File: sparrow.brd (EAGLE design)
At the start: 80 x 80 mm, 201 parts, among them IC1 LAN8720AVIAS, IC2 TLV320AIC3100VIAS, IC3 TPS2500, IC4 SKYWORKS_AAT4280ASC70JW-8-NOT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, IC5 SKYWORKS_AAT4280ASC70JW-8-NOT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, IC6 SKYWORKS_AAT4280ASC70JW-8-NOT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, IC7 SKYWORKS_AAT4280ASC70JW-8-NOT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, IC8 SKYWORKS_AAT4280ASC70JW-8-NOT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, IC9 FXMA10820-DFN, X1 ABS07-32768, X2 12MHz, X3 32768, X4 50MHZ, X5 16MHz

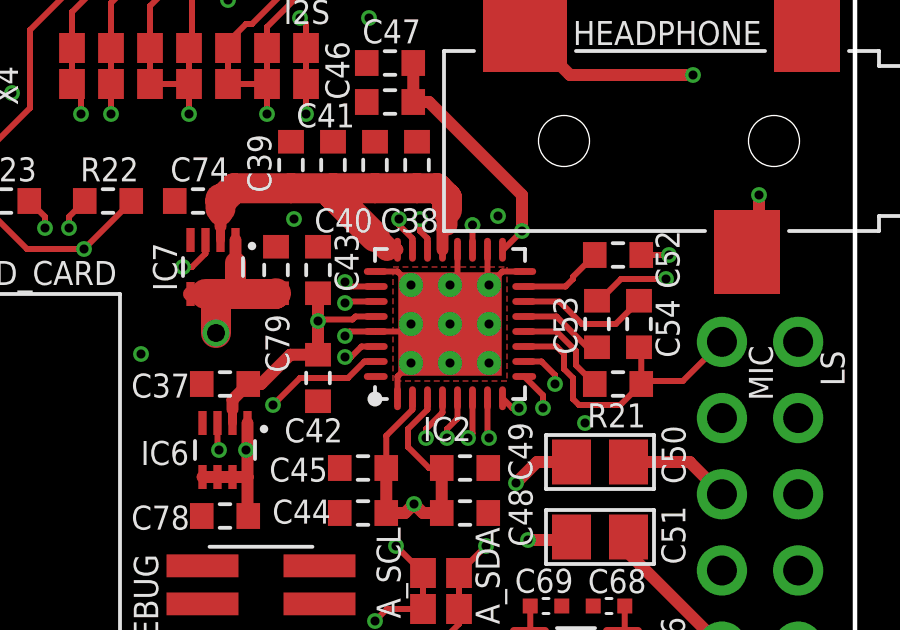
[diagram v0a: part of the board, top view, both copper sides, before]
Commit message: Last library update, DRC fixes
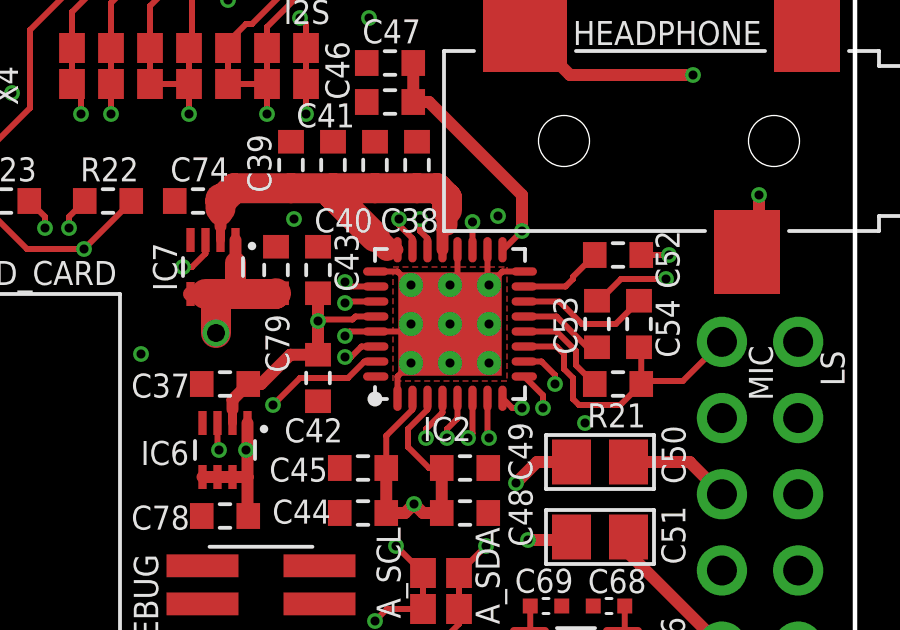
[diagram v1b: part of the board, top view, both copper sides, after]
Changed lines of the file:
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@@
 <contactref element="IC2" pad="19"/>
 <contactref element="LS" pad="2"/>
-<wire x1="67.25" y1="30.375" x2="67.25" y2="31.2" width="0.2" layer="1"/>
-<via x="67.25" y="31.2" extent="1-16" drill="0.3"/>
+<wire x1="67.25" y1="30.375" x2="67.25" y2="31.3" width="0.2" layer="1"/>
+<via x="67.25" y="31.3" extent="1-16" drill="0.3"/>
 <via x="64.8" y="31.4" extent="1-16" drill="0.3"/>
 <wire x1="65.25" y1="30.375" x2="65.25" y2="30.75" width="0.2" layer="1"/>
@@
 <wire x1="64.8" y1="31" x2="65.4" y2="30.4" width="0.4" layer="2"/>
 <wire x1="65.4" y1="30.4" x2="66.45" y2="30.4" width="0.4" layer="2"/>
-<wire x1="66.45" y1="30.4" x2="67.25" y2="31.2" width="0.4" layer="2"/>
 <wire x1="67.8" y1="32.2" x2="67.25" y2="31.65" width="0.4" layer="15"/>
-<wire x1="67.25" y1="31.65" x2="67.25" y2="31.2" width="0.4" layer="15"/>
+<wire x1="67.25" y1="31.65" x2="67.25" y2="31.3" width="0.4" layer="15"/>
 <wire x1="73.6" y1="31.8" x2="68.9" y2="31.8" width="0.4" layer="15"/>
 <wire x1="68.9" y1="31.8" x2="68.5" y2="32.2" width="0.4" layer="15"/>
@@
 <wire x1="76.8" y1="28.6" x2="76.8" y2="26.07" width="0.4" layer="15"/>
 <wire x1="76.8" y1="26.07" x2="78.105" y2="24.765" width="0.4" layer="15"/>
+<wire x1="66.45" y1="30.4" x2="67.25" y2="31.2" width="0.4" layer="2"/>
+<wire x1="67.25" y1="31.2" x2="67.25" y2="31.3" width="0.4" layer="2"/>
 </signal>
 <signal name="HPR">
@@
 <contactref element="MCLK" pad="2"/>
 <wire x1="68.25" y1="25.425" x2="68.575" y2="25.1" width="0.2" layer="1"/>
-<wire x1="68.575" y1="25.1" x2="68.8" y2="25.1" width="0.2" layer="1"/>
-<via x="68.8" y="25.1" extent="1-16" drill="0.3"/>
-<wire x1="68.8" y1="25.1" x2="67.7" y2="25.1" width="0.2" layer="15"/>
+<wire x1="68.575" y1="25.1" x2="68.9" y2="25.1" width="0.2" layer="1"/>
+<via x="68.9" y="25.1" extent="1-16" drill="0.3"/>
+<wire x1="68.9" y1="25.1" x2="67.7" y2="25.1" width="0.2" layer="15"/>
 <wire x1="67.7" y1="25.1" x2="67" y2="25.8" width="0.2" layer="15"/>
 <wire x1="67" y1="25.8" x2="63.2" y2="25.8" width="0.2" layer="15"/>

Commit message: Updated values
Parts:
- C10, C8, C9: value 4µ7 -> 4.7u
- C27, C52, C53, C56, C76, C77, C78, C79, C80: value 1µ -> 1u
- C29, C42, C44, C46, C48, L1: value 10µ -> 10u
- C40, C41: value 22µ -> 22u
- C50, C51: value 47µ -> 47u
- C55: value 2p2 -> 2.2p
- C57, C59: value 22µ 10V -> 22u 10V
- C60: value 150µ 10V -> 150u 10V
- C72, L5: value 2n2 -> 2.2n
- L7: value 2µ2 -> 2.2u
- R1: value 768k -> 768K
- R10, R11, R12, R13, R8, R9: value 12K -> 10K
- R16: value 12K1 -> 12.1K
- R17, R18, R19, R20: value 49R9 -> 49.9 1%
- R2: value 2M4 -> 2.4M
- R21, R22, R23, R38, R39: value 2K2 -> 2.2K
- R26: value 40K2 -> 40.2K
- R7: value 12K -> 12K 1%

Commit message: value tuning
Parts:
- R4, R43, R44, R45: value 806 -> 1K
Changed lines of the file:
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@@
 <attribute name="NAME" x="69.278" y="58.354" size="0.8" layer="25" font="vector"/>
 </element>
-<element name="R4" library="everykey" package="0603" value="806" x="69.4" y="55.4" smashed="yes" rot="R90">
+<element name="R4" library="everykey" package="0603" value="1K" x="69.4" y="55.4" smashed="yes" rot="R90">
 <attribute name="NAME" x="70.446" y="54.878" size="0.5" layer="25" font="vector" rot="R90"/>
 </element>
@@
 <attribute name="NAME" x="69.2" y="42.9" size="0.8" layer="25" font="vector" rot="R90"/>
 </element>
-<element name="R43" library="everykey" package="0603" value="806" x="32.5" y="70.6" smashed="yes" rot="R180">
+<element name="R43" library="everykey" package="0603" value="1K" x="32.5" y="70.6" smashed="yes" rot="R180">
 <attribute name="NAME" x="33.854" y="69.822" size="0.8" layer="25" font="vector" rot="R270"/>
 </element>
-<element name="R44" library="everykey" package="0603" value="806" x="32.5" y="69.1" smashed="yes" rot="R180">
+<element name="R44" library="everykey" package="0603" value="1K" x="32.5" y="69.1" smashed="yes" rot="R180">
 <attribute name="NAME" x="33.854" y="72.122" size="0.8" layer="25" font="vector" rot="R270"/>
 </element>
-<element name="R45" library="everykey" package="0603" value="806" x="32.5" y="72.1" smashed="yes" rot="R180">
+<element name="R45" library="everykey" package="0603" value="1K" x="32.5" y="72.1" smashed="yes" rot="R180">
 <attribute name="NAME" x="31.578" y="72.854" size="0.8" layer="25" font="vector"/>
 </element>
